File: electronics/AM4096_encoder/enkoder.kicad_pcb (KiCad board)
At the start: 2 copper layers, 42 x 42 mm, 16 parts, among them J1 Conn_01x04, J2 Conn_01x04, U1 am4096

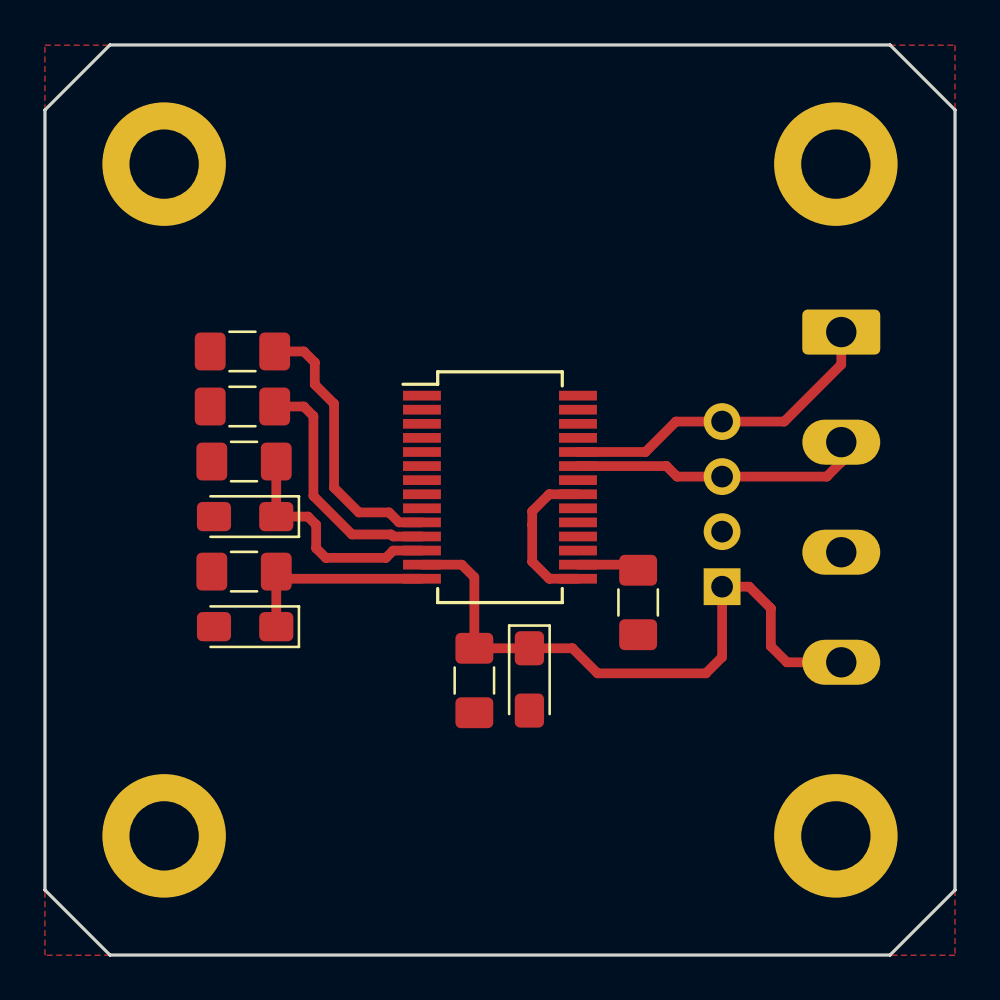
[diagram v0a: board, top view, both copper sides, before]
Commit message: Finish AM4096 encoder board
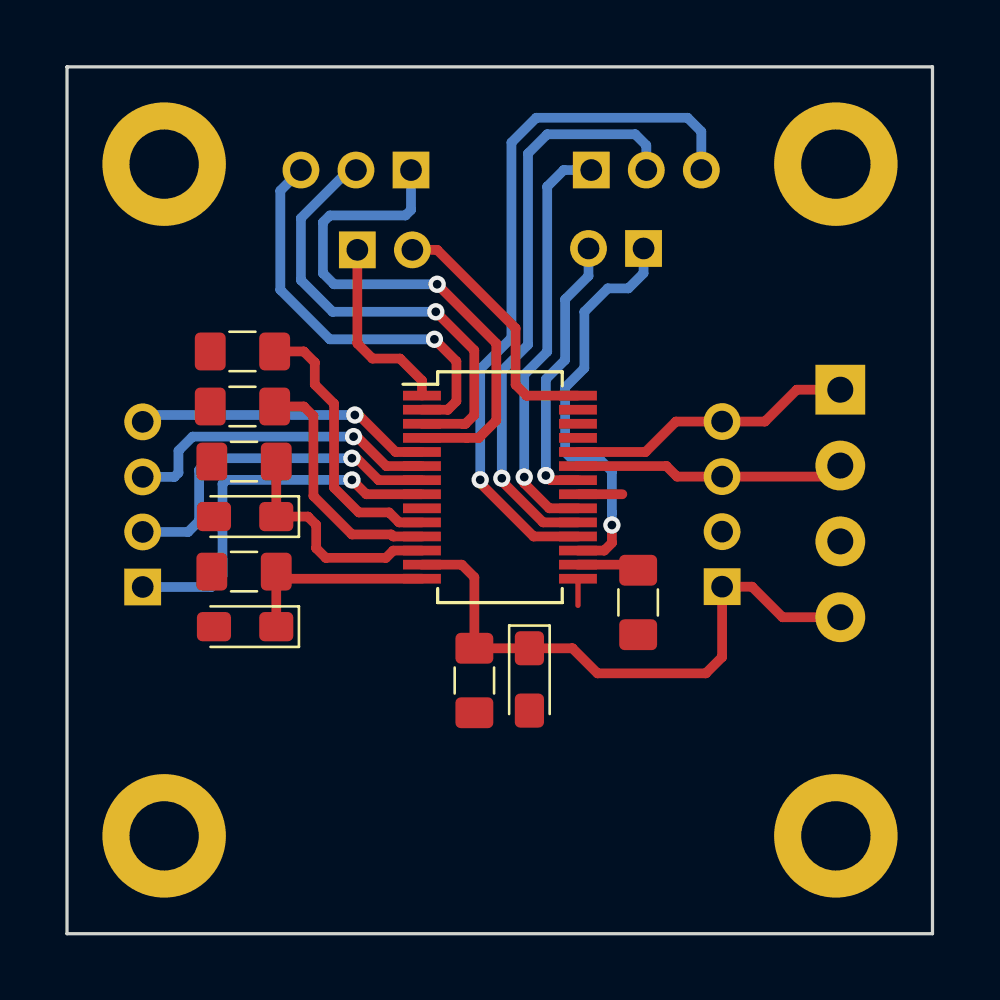
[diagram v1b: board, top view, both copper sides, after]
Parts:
- added J3: Conn_01x03, Connector_PinSocket_2.54mm:PinSocket_1x03_P2.54mm_Vertical, B.Cu at (159.9, 88.8)
- added J4: Conn_01x04, Connector_PinSocket_2.54mm:PinSocket_1x04_P2.54mm_Vertical, B.Cu at (147.5, 108.0)
- added J5: Conn_01x02, Connector_PinSocket_2.54mm:PinSocket_1x02_P2.54mm_Vertical, B.Cu at (157.4, 92.5)
- added J6: Conn_01x03, Connector_PinSocket_2.54mm:PinSocket_1x03_P2.54mm_Vertical, B.Cu at (168.2, 88.8)
- added J7: Conn_01x02, Connector_PinSocket_2.54mm:PinSocket_1x02_P2.54mm_Vertical, B.Cu at (170.6, 92.4)
- J2: footprint Connector_Phoenix_MSTB:PhoenixContact_MSTBA_2,5_4-G-5,08_1x04_P5.08mm_Horizontal -> TerminalBlock_MetzConnect:TerminalBlock_MetzConnect_Type059_RT06304HBWC_1x04_P3.50mm_Horizontal
- moved J2 2.66 mm to (179.7, 98.9)
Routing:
- net Net-(J6-Pad3): track 0.00 -> 33.1 mm, vias 0 -> 1
- net Net-(J6-Pad2): track 0.00 -> 27.1 mm, vias 0 -> 1
- net Net-(J3-Pad1): track 0.00 -> 25.2 mm, vias 0 -> 1
- net Net-(J3-Pad2): track 0.00 -> 21.2 mm, vias 0 -> 1
- net Net-(J6-Pad1): track 0.00 -> 19.4 mm, vias 0 -> 1
- net Net-(J3-Pad3): track 0.00 -> 19.0 mm, vias 0 -> 1
- net Net-(J7-Pad1): track 0.00 -> 19.0 mm, vias 0 -> 1
- net Net-(J4-Pad1): track 0.00 -> 17.7 mm, vias 0 -> 1
- net Net-(J4-Pad2): track 0.00 -> 16.1 mm, vias 0 -> 1
- net Net-(J4-Pad3): track 0.00 -> 14.8 mm, vias 0 -> 1
- net Net-(J4-Pad4): track 0.00 -> 13.7 mm, vias 0 -> 1
- net Net-(J7-Pad2): track 0.00 -> 12.9 mm, vias 0 -> 1
- net Net-(J5-Pad2): track 0.00 -> 12.0 mm
- net Net-(J5-Pad1): track 0.00 -> 8.71 mm
- net GND: track 7.39 -> 3.47 mm
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- added copper zone on B.Cu, net GND
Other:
- board size 42 x 42 mm -> 39.9 x 40 mm
- board text added: "A"
- board text added: "B"
- board text added: "Clock"
- board text added: "Data"
- board text added: "Mag"
- board text added: "RefN"
- board text added: "RefP"
- board text added: "Ri"
- board text added: "Td"
- board text added: "U"
- board text added: "V"
- board text added: "Vout"
- board text added: "W"
- board text added: "Zero"
- board text removed: "AM4096 Angular magnetic encoder for NEMA17 stepper motor"
